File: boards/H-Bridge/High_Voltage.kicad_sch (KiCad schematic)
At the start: 22 parts, among them IC2 MIC4606-1YML-TR, IC3 AD8410AWBRZ-RL, J1 V+, J2 V-, J3 Motor-, J4 Motor+, J9 12V+, M1 Motor_DC, Q1 NTBLS4D0N15MC, Q2 NTBLS4D0N15MC, Q3 NTBLS4D0N15MC, Q4 NTBLS4D0N15MC

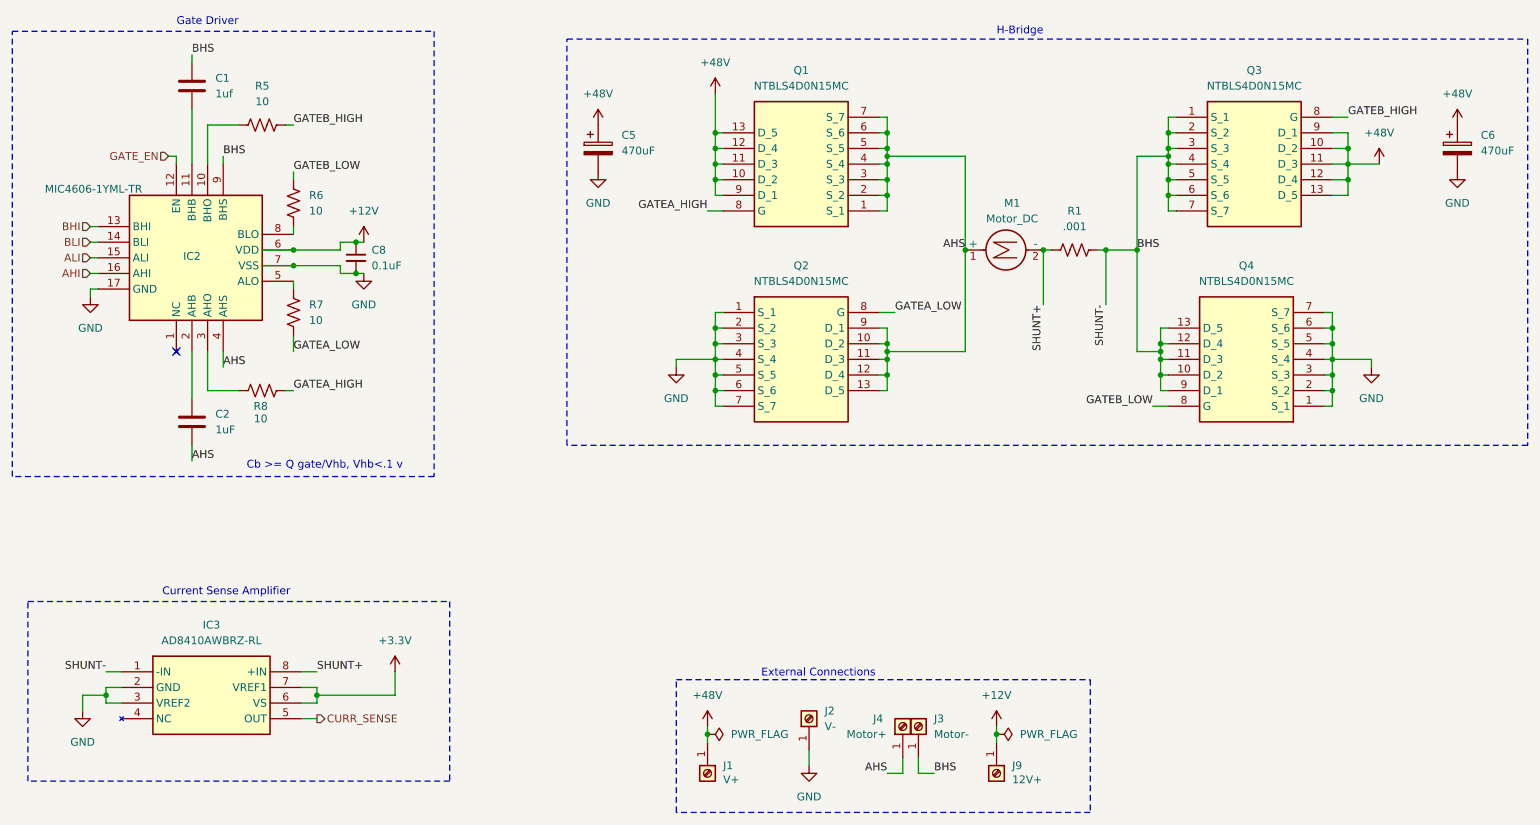
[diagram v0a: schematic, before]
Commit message: finished schematic, added footprint assignments
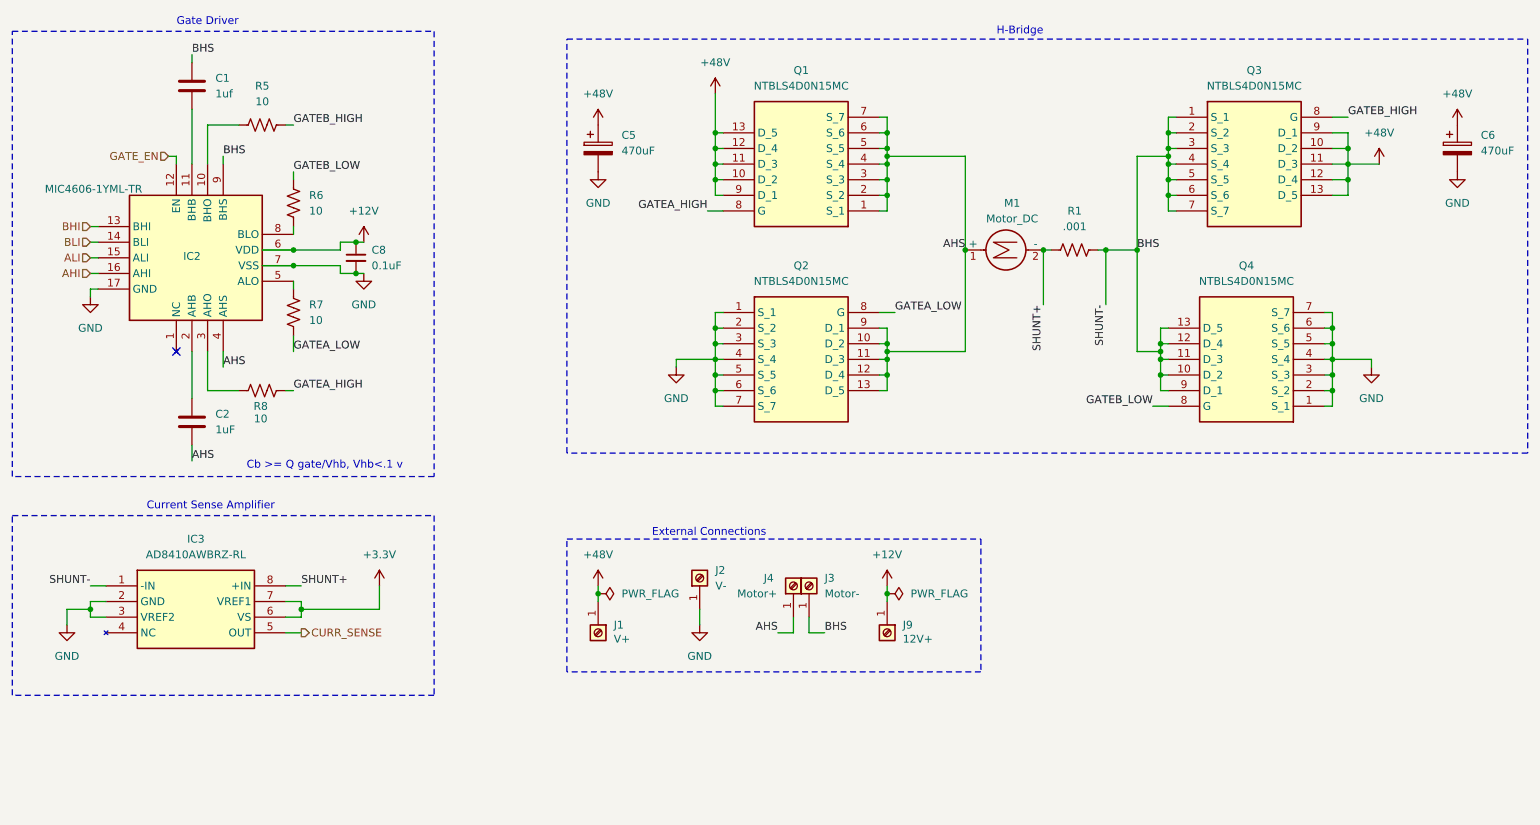
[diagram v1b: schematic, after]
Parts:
- C1, C2: footprint (none) -> Capacitor_SMD:C_0603_1608Metric
- C5, C6: footprint (none) -> Capacitor_THT:CP_Radial_D10.0mm_P7.50mm
- C8: footprint (none) -> Capacitor_SMD:C_0402_1005Metric
- IC2: footprint QFN65P400X400X90-17N-D -> Package_DFN_QFN:QFN-16-1EP_4x4mm_P0.65mm_EP2.5x2.5mm
- IC3: footprint SOIC127P600X175-8N -> Package_SO:MSOP-8_3x3mm_P0.65mm
- R5, R6, R7, R8: footprint (none) -> Resistor_SMD:R_0603_1608Metric
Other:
- moved on the sheet: IC3, J1, J2, J3, J4, J9
